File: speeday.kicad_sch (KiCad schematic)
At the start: 1 part, among them U7 STM32F407VGTx

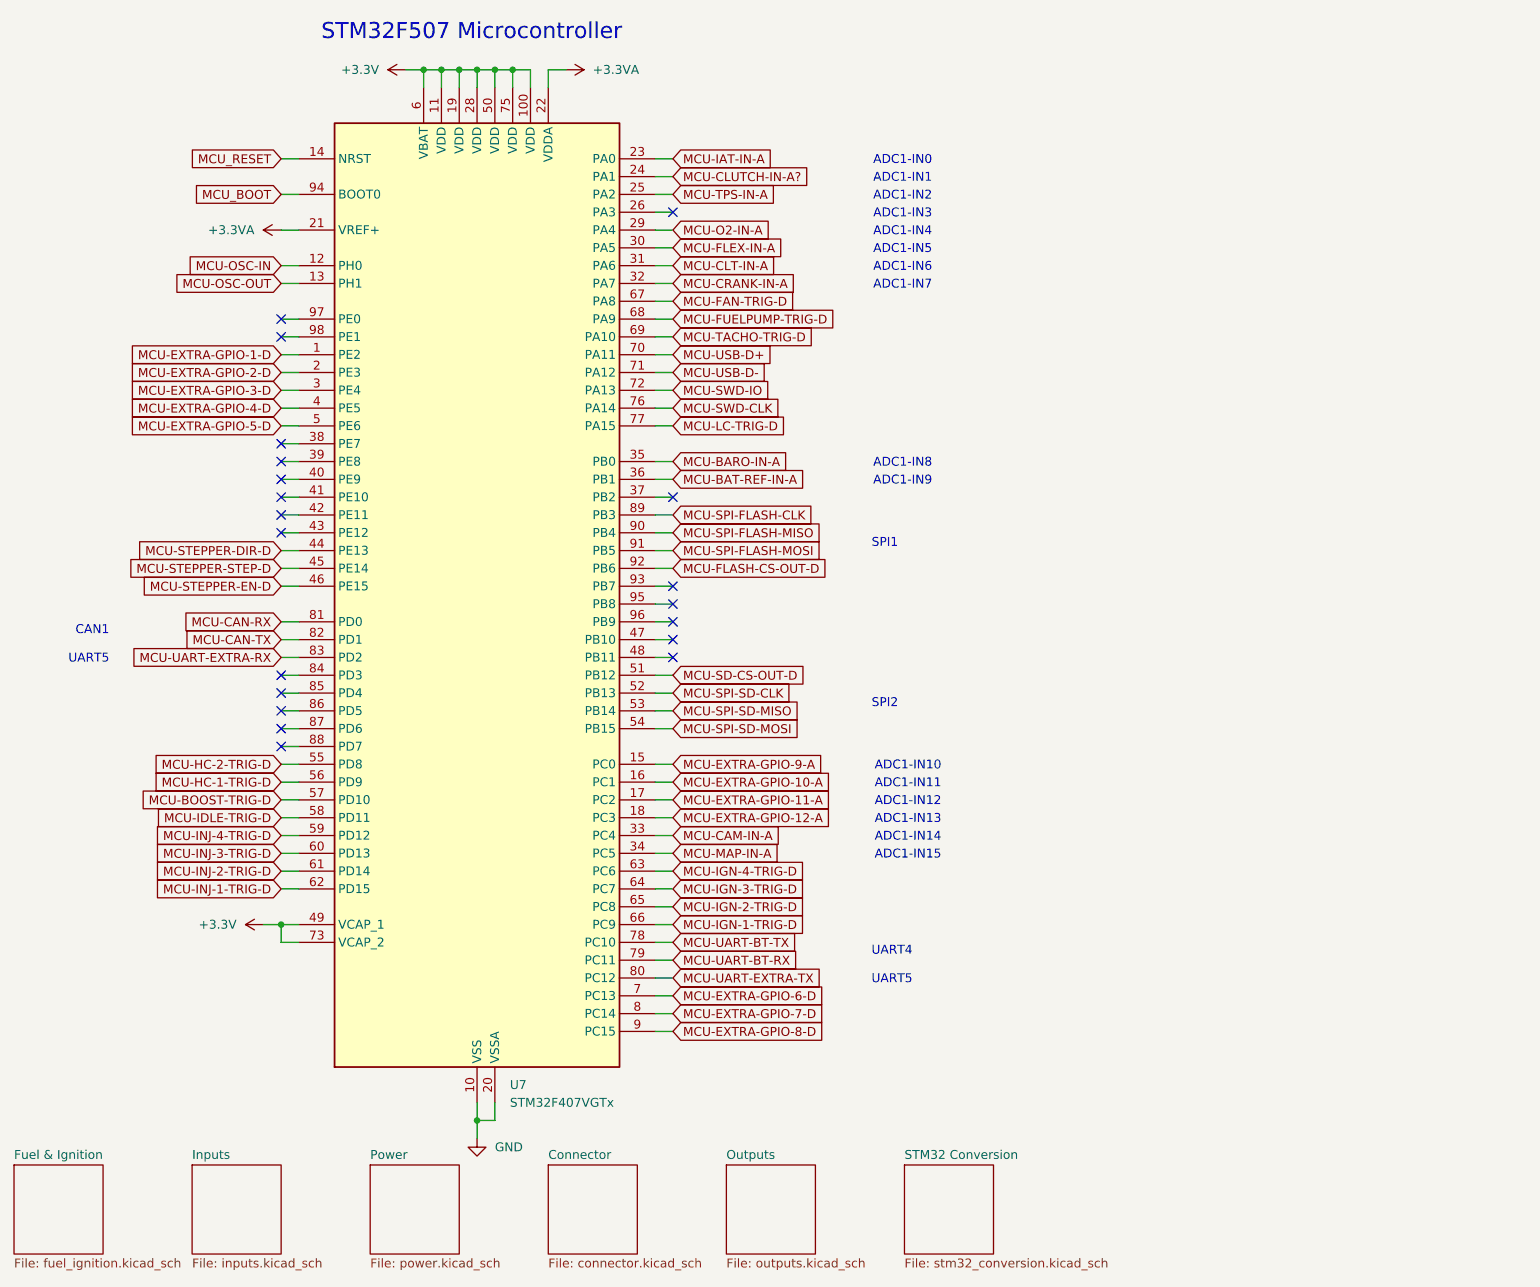
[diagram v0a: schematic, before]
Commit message: Fully connect all components
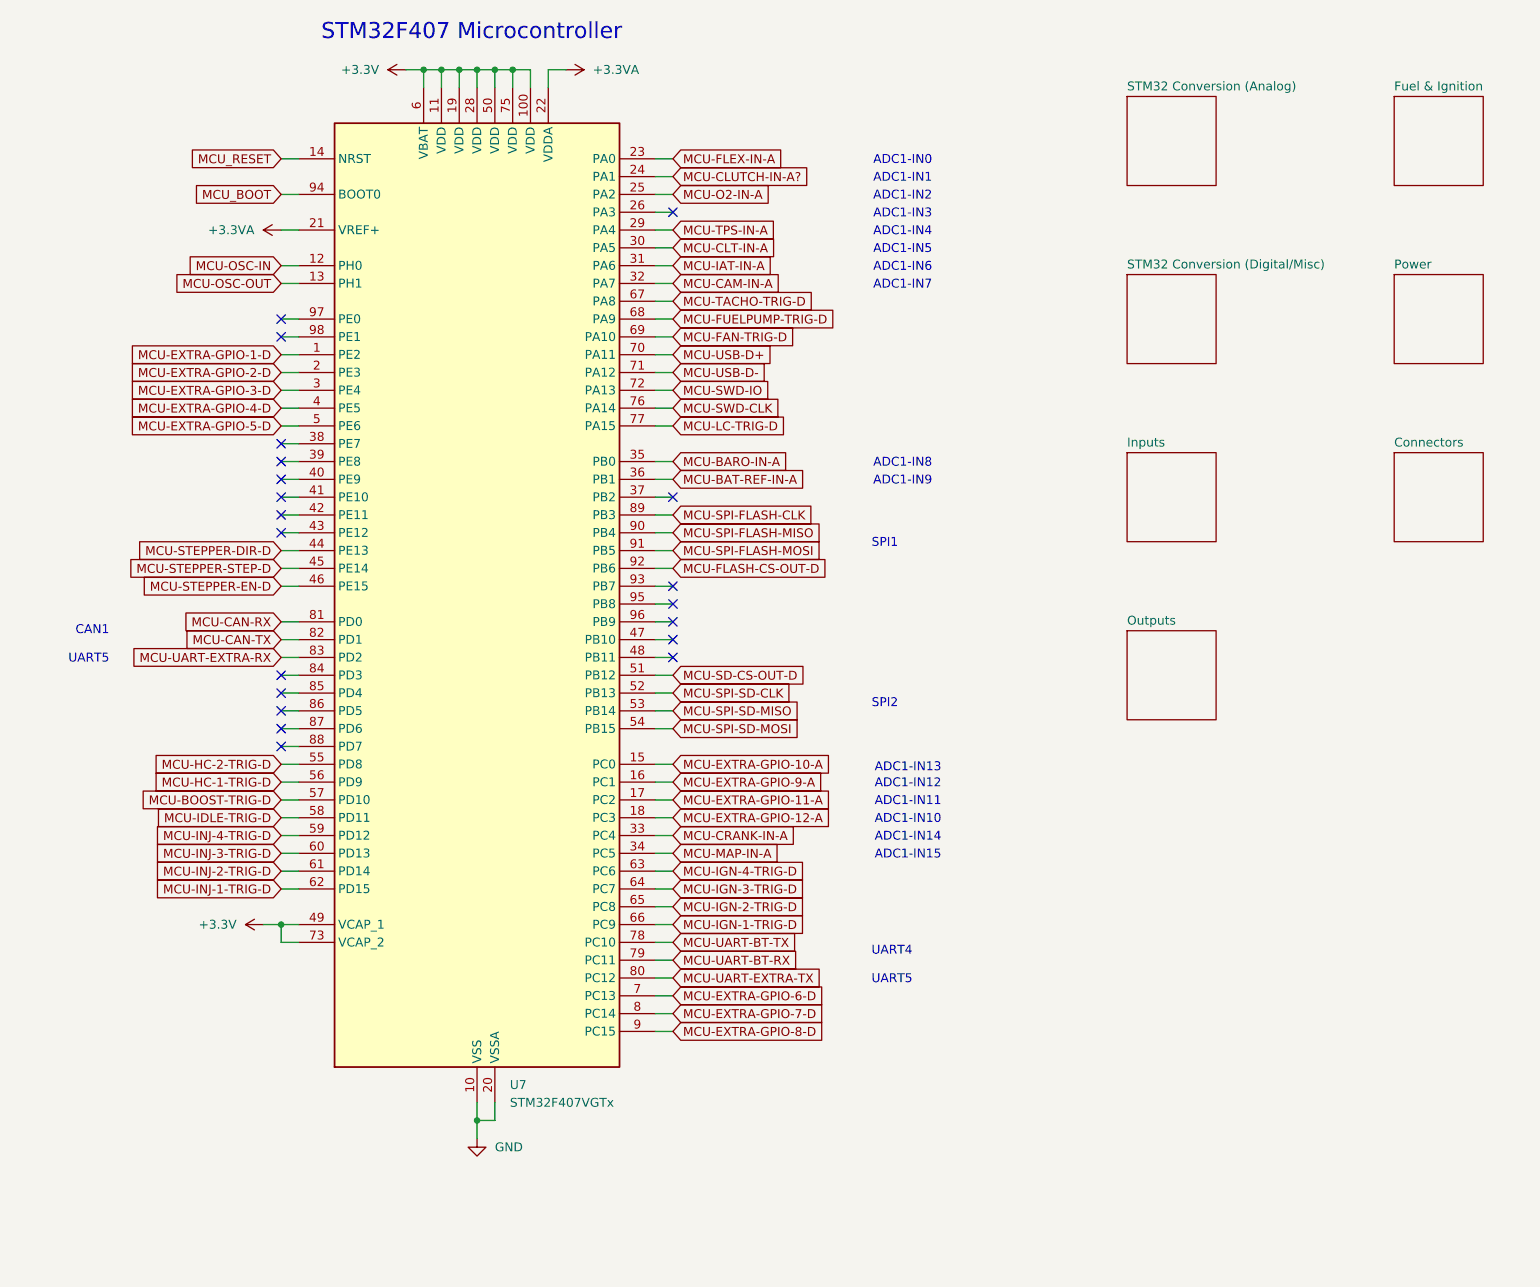
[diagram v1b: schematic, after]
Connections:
- net MCU-CAM-IN-A: now also U7.32 (PA7); no longer U7.33 (PC4)
- net MCU-CLT-IN-A: now also U7.30 (PA5); no longer U7.31 (PA6)
- net MCU-CRANK-IN-A: now also U7.33 (PC4); no longer U7.32 (PA7)
- net MCU-EXTRA-GPIO-10-A: now also U7.15 (PC0); no longer U7.16 (PC1)
- net MCU-EXTRA-GPIO-9-A: now also U7.16 (PC1); no longer U7.15 (PC0)
- net MCU-FAN-TRIG-D: now also U7.69 (PA10); no longer U7.67 (PA8)
- net MCU-FLEX-IN-A: now also U7.23 (PA0); no longer U7.30 (PA5)
- net MCU-IAT-IN-A: now also U7.31 (PA6); no longer U7.23 (PA0)
- net MCU-O2-IN-A: now also U7.25 (PA2); no longer U7.29 (PA4)
- net MCU-TACHO-TRIG-D: now also U7.67 (PA8); no longer U7.69 (PA10)
- net MCU-TPS-IN-A: now also U7.29 (PA4); no longer U7.25 (PA2)
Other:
- sheet Connector renamed Connectors
- sheet STM32 Conversion renamed STM32 Conversion (Analog)
- added sheet STM32 Conversion (Digital/Misc) (stm32_conversion_misc.kicad_sch)
- sheet Connectors: file connector.kicad_sch -> connectors.kicad_sch
- sheet STM32 Conversion (Analog): file stm32_conversion.kicad_sch -> stm32_conversion_analog_digital.kicad_sch
- note added: "STM32F407 Microcontroller"
- note removed: "STM32F507 Microcontroller"
